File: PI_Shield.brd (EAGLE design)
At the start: 78.7 x 69.5 mm, 64 parts, among them Q1 220mA/50V/3.5Ω, Q3 220mA/50V/3.5Ω, Q4 220mA/50V/3.5Ω, Q5 2.5A/30V/105mΩ, U1 MAX1136EUA-T, U2 AZ1117EH-3.3TRG1, Y1 ECS-80-S-4X

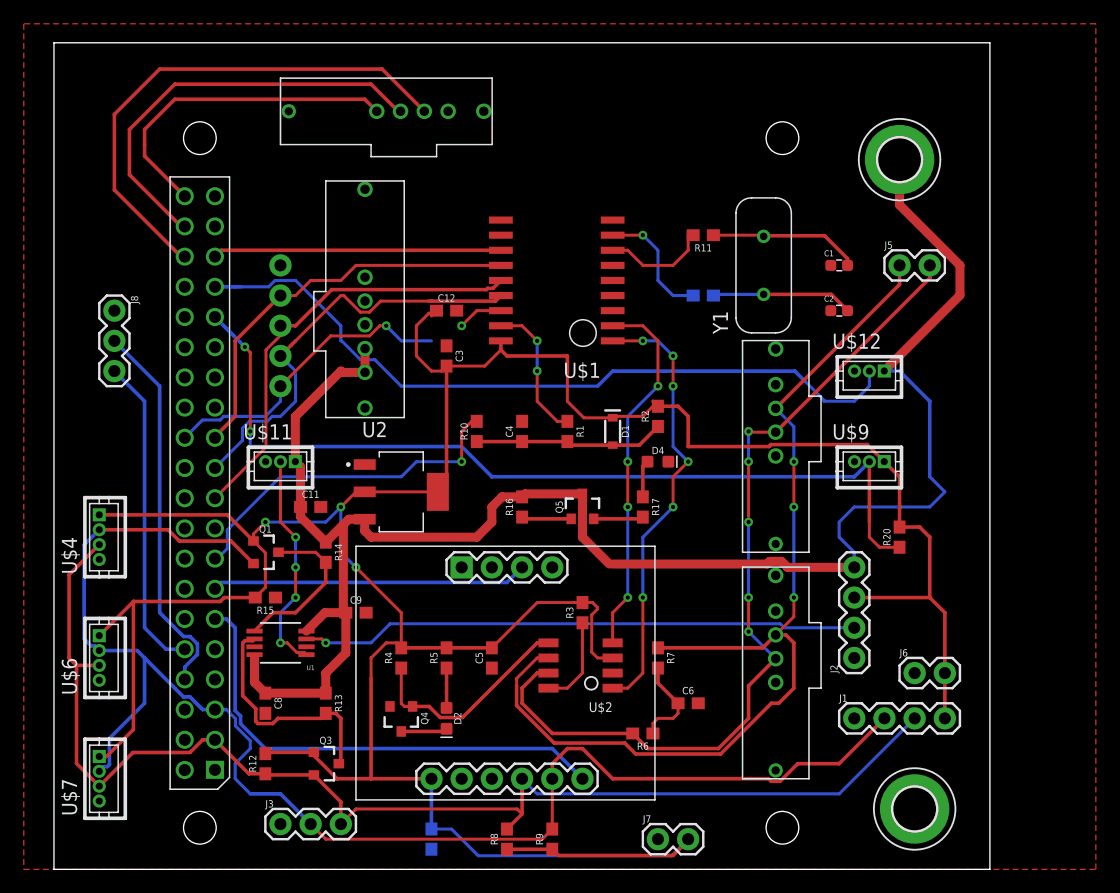
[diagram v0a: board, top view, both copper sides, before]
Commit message: Update PI_Shield.brd
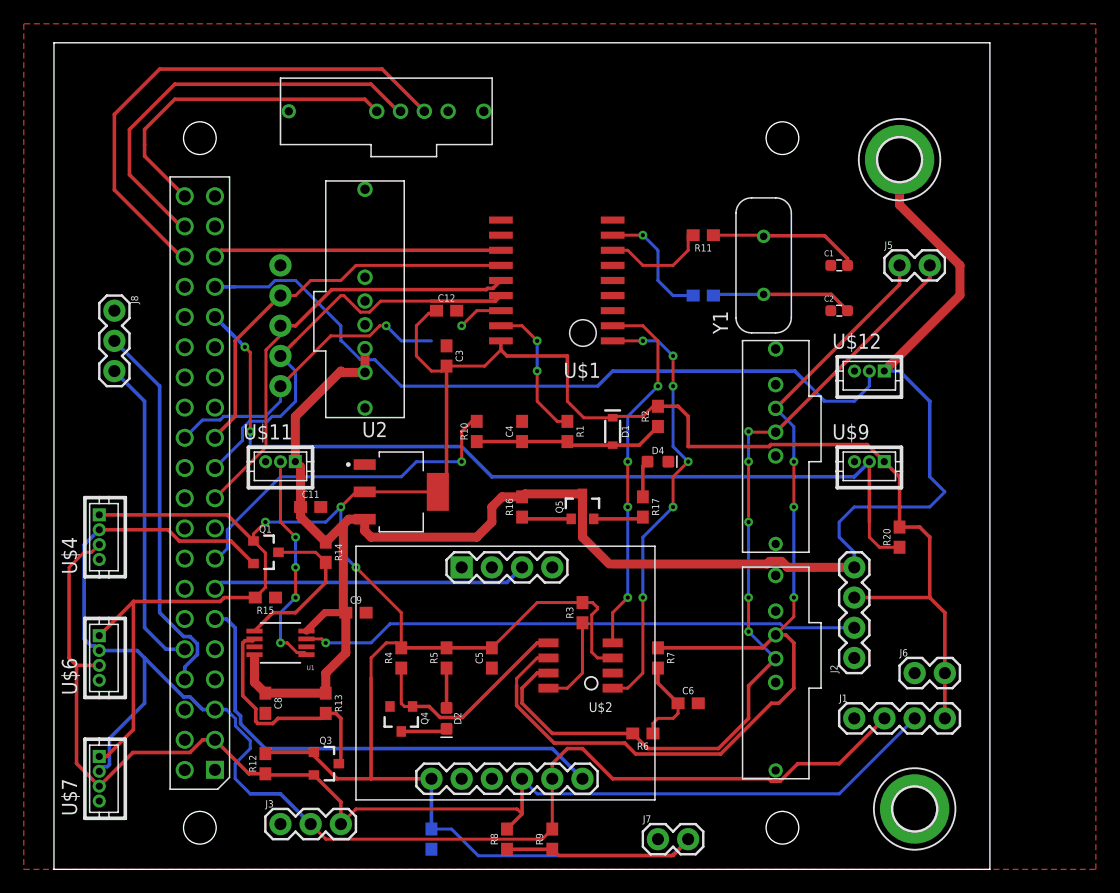
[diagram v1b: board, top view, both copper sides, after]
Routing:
- net 3V3: track 274.2 -> 272.9 mm
- net SDA: track 108.4 -> 107.5 mm
- net PWM: track 63.6 -> 63.1 mm
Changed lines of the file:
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@@
 <contactref element="C2" pad="2"/>
 <contactref element="Y1" pad="1"/>
-<wire x1="73.66" y1="57.25" x2="73.56" y2="57.15" width="0.3048" layer="1"/>
 <wire x1="73.66" y1="57.25" x2="79.345" y2="57.25" width="0.3048" layer="1"/>
 <wire x1="79.345" y1="57.25" x2="80.715" y2="55.88" width="0.3048" layer="1"/>
@@
 <wire x1="51.56" y1="57.15" x2="51.0948" y2="56.6848" width="0.3048" layer="1"/>
 <wire x1="51.0948" y1="56.6848" x2="45.72" y2="56.6848" width="0.3048" layer="1"/>
-<wire x1="45.72" y1="56.6848" x2="45.46375" y2="56.6848" width="0.3048" layer="1"/>
 <wire x1="33.02" y1="52.07" x2="34.29" y2="53.34" width="0.3048" layer="1"/>
 <wire x1="45.72" y1="56.6848" x2="41.44483125" y2="56.6848" width="0.254" layer="1"/>
@@
 <wire x1="31.85" y1="18.73" x2="31.75" y2="18.63" width="0.3048" layer="1"/>
 <wire x1="64.77" y1="47.84" x2="64.56" y2="48.05" width="0.3048" layer="1"/>
-<wire x1="64.56" y1="48.05" x2="64.35" y2="48.26" width="0.3048" layer="1"/>
-<wire x1="45.72" y1="55.46" x2="45.93" y2="55.67" width="0.3048" layer="1"/>
 <wire x1="45.93" y1="55.67" x2="46.14" y2="55.88" width="0.3048" layer="1"/>
 <wire x1="74.27285" y1="44.6188" x2="74.10405" y2="44.45" width="0.3048" layer="1"/>
@@
 <wire x1="45.72" y1="12.28" x2="47.41" y2="12.28" width="0.254" layer="16"/>
 <wire x1="47.41" y1="12.28" x2="48.26" y2="11.43" width="0.254" layer="16"/>
-<wire x1="48.26" y1="11.43" x2="49.53" y2="10.16" width="0.254" layer="16"/>
-<wire x1="49.53" y1="10.16" x2="49.657" y2="10.033" width="0.254" layer="16"/>
+<wire x1="48.26" y1="11.43" x2="49.657" y2="10.033" width="0.254" layer="16"/>
 <wire x1="65.913" y1="10.033" x2="67.31" y2="11.43" width="0.254" layer="16"/>
 <wire x1="49.657" y1="10.033" x2="65.913" y2="10.033" width="0.254" layer="16"/>
 <wire x1="50.8" y1="27.52" x2="54.61" y2="31.33" width="0.254" layer="1"/>
 <wire x1="54.61" y1="31.33" x2="58.42" y2="31.33" width="0.254" layer="1"/>
-<wire x1="58.84" y1="31.33" x2="58.42" y2="31.33" width="0.254" layer="1"/>
 <wire x1="30.75" y1="36.51" x2="31.75" y2="35.51" width="0.254" layer="1"/>
 <wire x1="31.75" y1="32.6" x2="30.9" y2="31.75" width="0.254" layer="1"/>
@@
 <wire x1="50.2" y1="51.22" x2="51.56" y2="52.58" width="0.254" layer="1"/>
 <wire x1="60.96" y1="26.67" x2="59.69" y2="26.67" width="0.254" layer="1"/>
-<wire x1="58.42" y1="31.07513125" x2="58.42" y2="31.33" width="0.254" layer="1"/>
 <wire x1="59.69" y1="26.67" x2="59.1994" y2="27.1606" width="0.254" layer="1"/>
 <wire x1="59.1994" y1="30.29573125" x2="59.1994" y2="27.1606" width="0.254" layer="1"/>
-<wire x1="58.42" y1="31.33" x2="59.27" y2="31.33" width="0.254" layer="1"/>
 <wire x1="59.69" y1="30.78633125" x2="59.1994" y2="30.29573125" width="0.254" layer="1"/>
-<wire x1="59.27" y1="31.33" x2="59.69" y2="30.91" width="0.254" layer="1"/>
+<wire x1="59.69" y1="30.91" x2="59.27" y2="31.33" width="0.254" layer="1"/>
 <wire x1="59.69" y1="30.91" x2="59.69" y2="30.78633125" width="0.254" layer="1"/>
 <wire x1="43.18" y1="27.52" x2="42.76" y2="27.94" width="0.254" layer="1"/>
@@
 <wire x1="44.45" y1="54.61" x2="45.51" y2="55.67" width="0.254" layer="1"/>
 <wire x1="45.51" y1="55.67" x2="45.93" y2="55.67" width="0.254" layer="1"/>
-<wire x1="48.26" y1="11.43" x2="48.26" y2="11.43" width="0.254" layer="16"/>
+<wire x1="59.27" y1="31.33" x2="58.42" y2="31.33" width="0.254" layer="1"/>
 </signal>
 <signal name="N$1">
@@
 <contactref element="R6" pad="1"/>
 <contactref element="R7" pad="2"/>
-<wire x1="66.46" y1="22.86" x2="66.46" y2="22.43" width="0.3048" layer="1"/>
 <wire x1="66.46" y1="22.86" x2="64.77" y2="24.55" width="0.3048" layer="1"/>
 <wire x1="64.77" y1="24.55" x2="64.77" y2="25.82" width="0.3048" layer="1"/>
-<wire x1="66.46" y1="22.86" x2="66.46" y2="22.01" width="0.254" layer="1"/>
-<wire x1="66.46" y1="22.01" x2="66.04" y2="21.59" width="0.254" layer="1"/>
-<wire x1="66.04" y1="21.59" x2="64.77" y2="21.59" width="0.254" layer="1"/>
+<wire x1="64.77" y1="21.59" x2="66.04" y2="21.59" width="0.254" layer="1"/>
 <wire x1="64.77" y1="21.59" x2="64.35" y2="21.17" width="0.254" layer="1"/>
 <wire x1="64.35" y1="21.17" x2="64.35" y2="20.32" width="0.254" layer="1"/>
+<wire x1="66.04" y1="21.59" x2="66.46" y2="22.01" width="0.254" layer="1"/>
+<wire x1="66.46" y1="22.01" x2="66.46" y2="22.86" width="0.254" layer="1"/>
 </signal>
 <signal name="DI1">
@@
 <contactref element="Q3" pad="2"/>
 <contactref element="R12" pad="1"/>
-<wire x1="53.34" y1="15.24" x2="53.34" y2="16.51" width="0.3048" layer="1"/>
 <wire x1="53.34" y1="16.51" x2="53.34" y2="13.55" width="0.3048" layer="1"/>
 <wire x1="53.34" y1="13.55" x2="52.07" y2="12.28" width="0.3048" layer="1"/>
@@
 <wire x1="20.6148" y1="18.7198" x2="17.78" y2="15.885" width="0.3048" layer="1"/>
 <wire x1="25.4100875" y1="18.7198" x2="20.6148" y2="18.7198" width="0.3048" layer="1"/>
-<wire x1="17.78" y1="36.205" x2="15.24" y2="33.665" width="0.3048" layer="1"/>
 <wire x1="15.24" y1="33.665" x2="15.24" y2="26.67" width="0.3048" layer="1"/>
 <wire x1="15.24" y1="26.67" x2="15.865" y2="26.045" width="0.3048" layer="1"/>
@@
 <wire x1="54.61" y1="15.24" x2="53.34" y2="16.51" width="0.254" layer="16"/>
 <wire x1="80.01" y1="15.24" x2="54.61" y2="15.24" width="0.254" layer="16"/>
+<wire x1="17.78" y1="36.205" x2="17.135" y2="35.56" width="0.254" layer="1"/>
+<wire x1="17.135" y1="35.56" x2="16.51" y2="35.56" width="0.254" layer="1"/>
+<wire x1="16.51" y1="35.56" x2="15.24" y2="34.29" width="0.254" layer="1"/>
+<wire x1="15.24" y1="34.29" x2="15.24" y2="33.665" width="0.254" layer="1"/>
 </signal>
 <signal name="SCL">
@@
 <wire x1="87.63" y1="48.26" x2="85.085" y2="50.805" width="0.3048" layer="16"/>
 <wire x1="85.085" y1="50.805" x2="83.8" y2="50.805" width="0.3048" layer="16"/>
-<wire x1="81.0012" y1="34.5688" x2="81.28" y2="34.29" width="0.3048" layer="1"/>
 <wire x1="60.6812" y1="34.5688" x2="60.96" y2="34.5688" width="0.3048" layer="1"/>
 <wire x1="36.83" y1="23.71" x2="31.75" y2="23.71" width="0.762" layer="1"/>
@@
 <wire x1="38.52" y1="27.09" x2="38.52" y2="30.48" width="0.762" layer="1"/>
 <wire x1="36.83" y1="25.4" x2="38.52" y2="27.09" width="0.762" layer="1"/>
-<wire x1="35.2044" y1="28.9306" x2="36.7538" y2="30.48" width="0.762" layer="1"/>
-<wire x1="36.7538" y1="30.48" x2="38.52" y2="30.48" width="0.762" layer="1"/>
 <wire x1="38.52" y1="30.48" x2="38.31" y2="30.69" width="0.762" layer="1"/>
 <wire x1="38.31" y1="30.69" x2="38.31" y2="37.89" width="0.762" layer="1"/>
@@
 <wire x1="80.01" y1="36.83" x2="81.28" y2="35.56" width="0.254" layer="16"/>
 <wire x1="87.63" y1="39.37" x2="81.28" y2="39.37" width="0.254" layer="16"/>
+<wire x1="35.2044" y1="28.9306" x2="36.7538" y2="30.48" width="0.6096" layer="1"/>
+<wire x1="36.7538" y1="30.48" x2="38.52" y2="30.48" width="0.6096" layer="1"/>
 </signal>
 <signal name="IMU_INT">
@@
 <contactref element="R20" pad="1"/>
 <contactref element="PCB1" pad="P$31"/>
-<wire x1="85.09" y1="35.98" x2="84.67" y2="35.98" width="0.3048" layer="1"/>
 <wire x1="82.55" y1="43.175" x2="82.55" y2="38.1" width="0.3048" layer="1"/>
 <wire x1="27.5082" y1="55.3466" x2="29.9974" y2="52.8574" width="0.3048" layer="16"/>
@@
 <wire x1="76.28046875" y1="50.795" x2="77.13426875" y2="49.9412" width="0.3048" layer="16"/>
 <wire x1="27.5082" y1="57.8866" x2="29.21" y2="57.8866" width="0.3048" layer="16"/>
-<wire x1="29.21" y1="57.8866" x2="29.7434" y2="57.8866" width="0.3048" layer="16"/>
-<wire x1="29.21" y1="57.8866" x2="32.0323875" y2="57.8866" width="0.254" layer="16"/>
 <wire x1="32.0323875" y1="57.8866" x2="32.5657875" y2="58.42" width="0.254" layer="16"/>
 <wire x1="43.18" y1="49.53" x2="59.695" y2="49.53" width="0.254" layer="16"/>
@@
 <wire x1="82.55" y1="49.53" x2="82.55" y2="50.795" width="0.254" layer="16"/>
 <wire x1="78.74" y1="48.26" x2="81.28" y2="48.26" width="0.254" layer="16"/>
+<wire x1="29.21" y1="57.8866" x2="32.0323875" y2="57.8866" width="0.254" layer="16"/>
 </signal>
 <signal name="TX">
@@
 <wire x1="30.8356" y1="28.9306" x2="32.385" y2="30.48" width="0.3048" layer="1"/>
 <wire x1="32.385" y1="30.48" x2="34.29" y2="30.48" width="0.3048" layer="1"/>
-<wire x1="32.85" y1="35.56" x2="33.02" y2="35.56" width="0.254" layer="1"/>
+<wire x1="35.98" y1="35.56" x2="36.83" y2="34.71" width="0.254" layer="1"/>
 <wire x1="32.85" y1="35.56" x2="35.98" y2="35.56" width="0.254" layer="1"/>
-<wire x1="35.98" y1="35.56" x2="36.83" y2="34.71" width="0.254" layer="1"/>
 </signal>
 <signal name="SDA_ADC">
